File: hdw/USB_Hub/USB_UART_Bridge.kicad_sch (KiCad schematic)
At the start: 40 parts

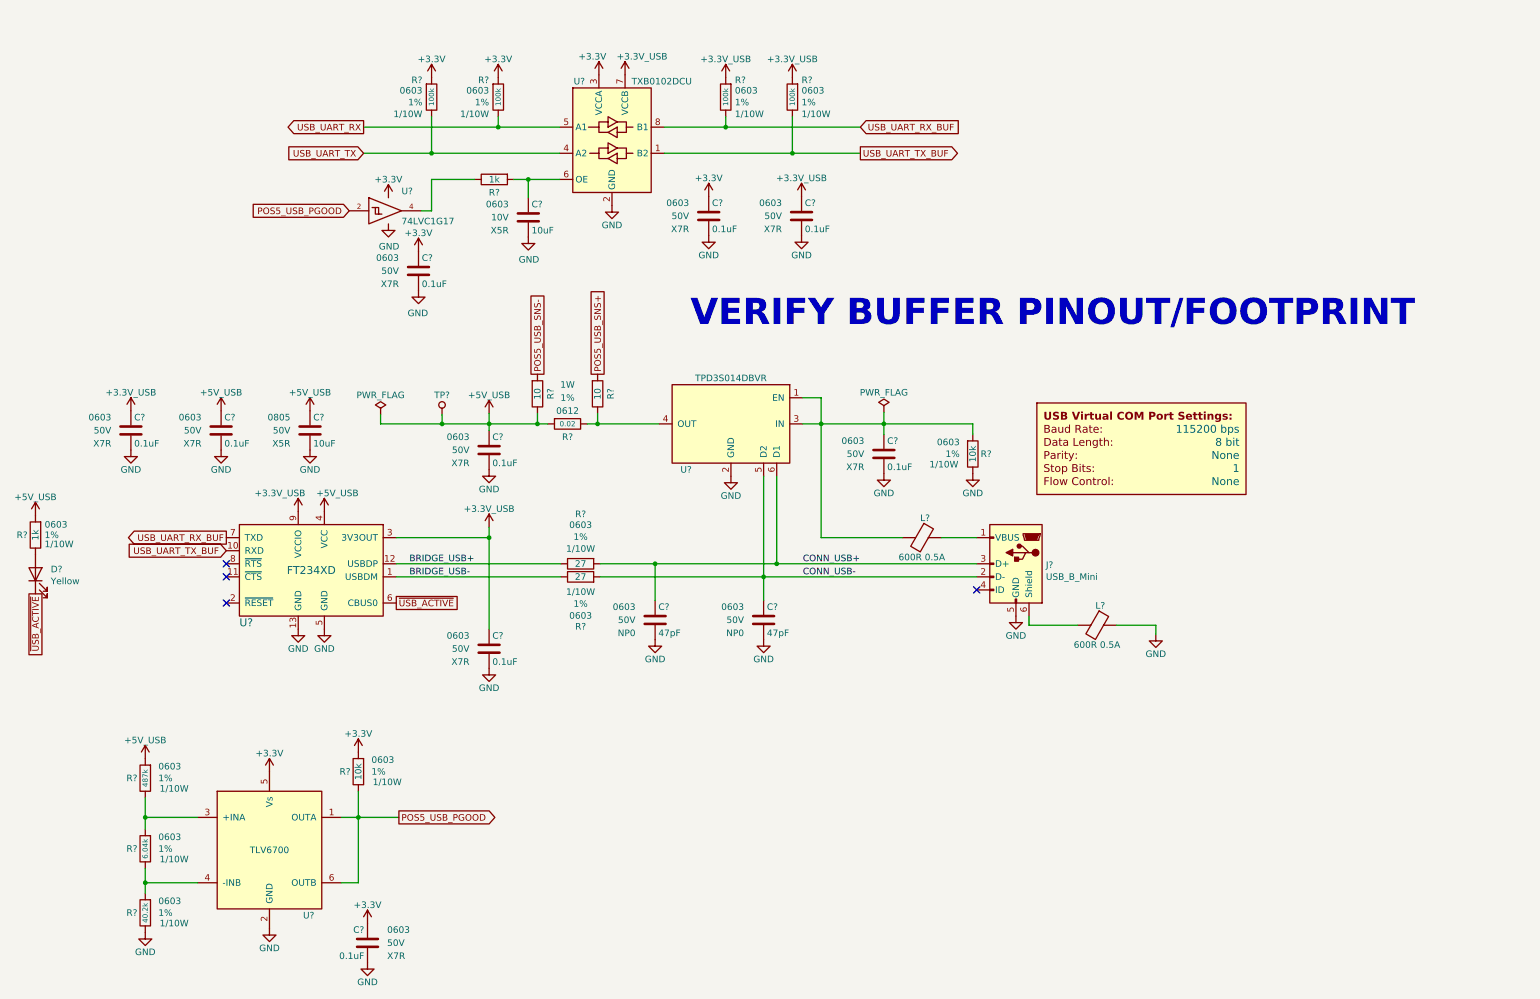
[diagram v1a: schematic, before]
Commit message: schematic progress
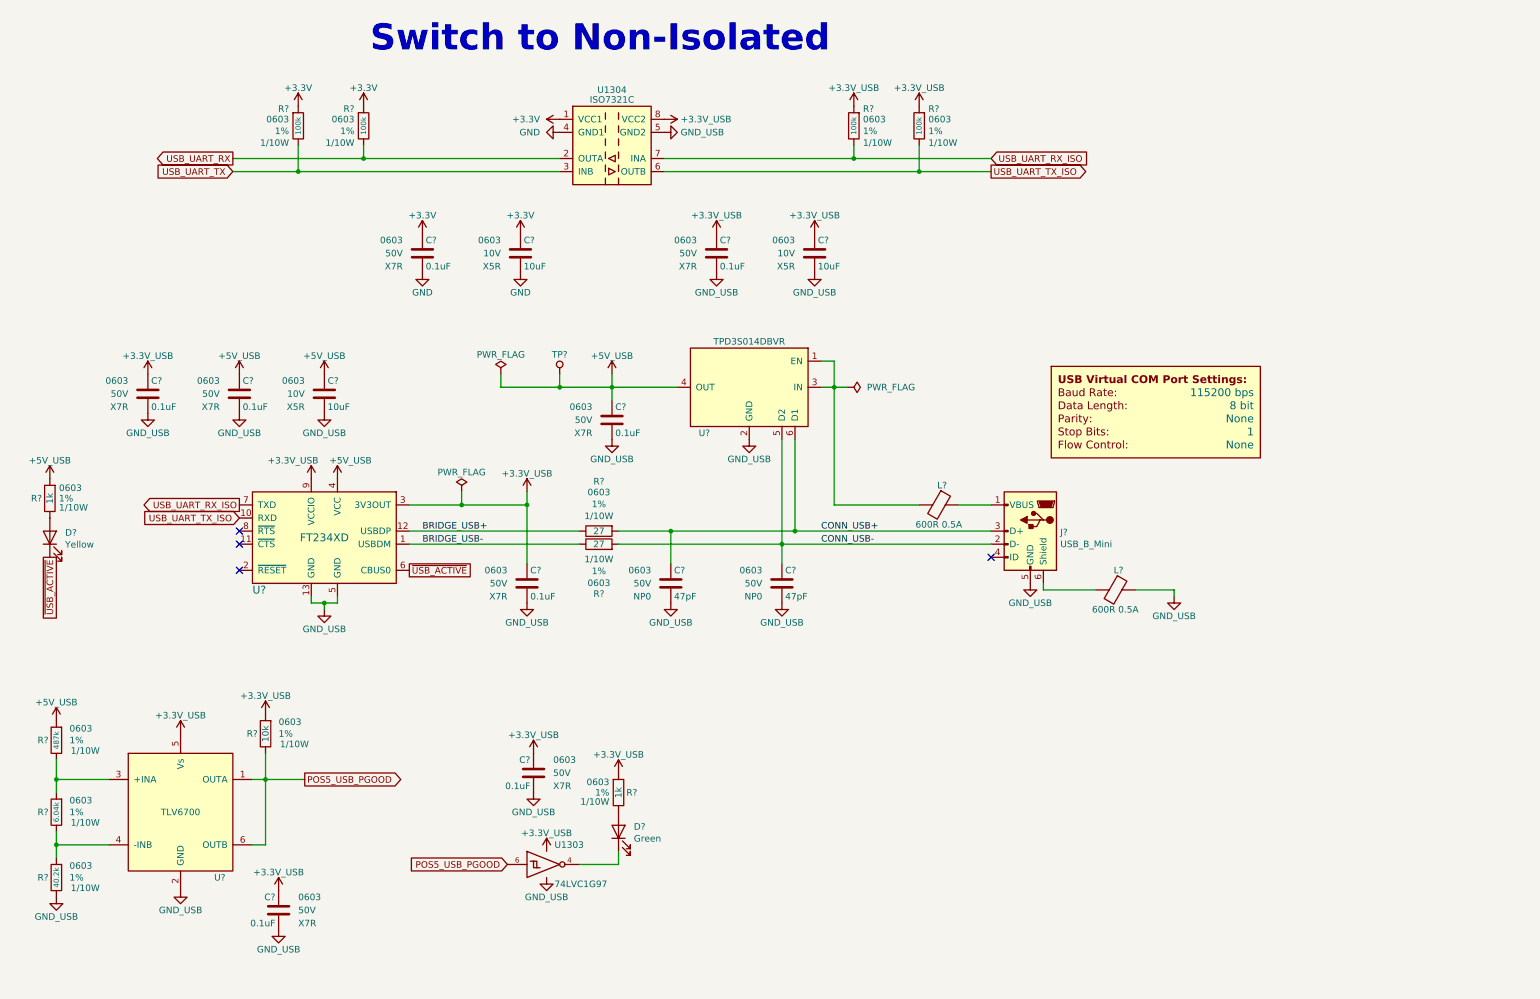
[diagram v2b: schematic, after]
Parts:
- removed C? (x2): 47pF, Capacitors_SMD:C_0603, symbol Custom_Library:C_Custom
- removed C? (x9): 0.1uF, Capacitors_SMD:C_0603, symbol Custom_Library:C_Custom
- removed C?: 10uF, Capacitors_SMD:C_0603, symbol Custom_Library:C_Custom
- removed C?: 10uF, Capacitors_SMD:C_0805, symbol Custom_Library:C_Custom
- removed D?: Yellow, LEDs:LED_0603, symbol Device:LED
- removed DOC?: COM_Port_Settings, symbol Custom_Library:COM_Port_Settings
- removed J?: USB_B_Mini, Connectors:USB_Mini-B, symbol Connector:USB_B_Mini
- removed L? (x2): 600R 0.5A, Inductors_SMD:L_0603, symbol Device:Ferrite_Bead
- removed R? (x2): 1k, Resistors_SMD:R_0603, symbol Custom_Library:R_Custom
- removed R? (x2): 27, Resistors_SMD:R_0603, symbol Custom_Library:R_Custom
- removed R?: 6.04k, Resistors_SMD:R_0603, symbol Custom_Library:R_Custom
- removed R?: 40.2k, Resistors_SMD:R_0603, symbol Custom_Library:R_Custom
- removed R?: 487k, Resistors_SMD:R_0603, symbol Custom_Library:R_Custom
- removed R? (x2): 10k, Resistors_SMD:R_0603, symbol Custom_Library:R_Custom
- removed R?: 0.02, Resistors_SMD:R_0612, symbol Custom_Library:R_Custom
- removed R? (x2): 10, Resistors_SMD:R_0603, symbol Custom_Library:R_Custom
- removed R? (x4): 100k, Resistors_SMD:R_0603, symbol Custom_Library:R_Custom
- removed TP?: TP, Custom Footprints Library:Test_Point, symbol Custom_Library:TP
- removed U?: FT234XD, Housings_DFN_QFN:DFN-12-1EP_3x3mm_Pitch0.45mm, symbol Custom_Library:FT234XD
- removed U?: TPD3S014DBVR, TO_SOT_Packages_SMD:SOT-23-6, symbol Custom_Library:TPD3S014DBVR
- removed U?: TLV6700, Package_TO_SOT_SMD:SOT-23-6, symbol Custom_Library:TLV6700
- removed U?: TXB0102DCU, Package_SO:VSSOP-8_2.4x2.1mm_P0.5mm, symbol Logic_LevelTranslator:TXB0102DCU
- removed U?: 74LVC1G17, TO_SOT_Packages_SMD:SOT-353_SC-70-5, symbol Custom_Library:74LVC1G17_Power
- added C? (x3): 10uF, Capacitors_SMD:C_0603, symbol Custom_Library:C_Custom
- added C? (x8): 0.1uF, Capacitors_SMD:C_0603, symbol Custom_Library:C_Custom
- added C? (x2): 47pF, Capacitors_SMD:C_0603, symbol Custom_Library:C_Custom
- added D?: Yellow, LEDs:LED_0603, symbol Device:LED
- added D?: Green, LEDs:LED_0603, symbol Device:LED
- added DOC?: COM_Port_Settings, symbol Custom_Library:COM_Port_Settings
- added J?: USB_B_Mini, Connectors:USB_Mini-B, symbol Connector:USB_B_Mini
- added L? (x2): 600R 0.5A, Inductors_SMD:L_0603, symbol Device:Ferrite_Bead
- added R? (x4): 100k, Resistors_SMD:R_0603, symbol Custom_Library:R_Custom
- added R?: 10k, Resistors_SMD:R_0603, symbol Custom_Library:R_Custom
- added R?: 487k, Resistors_SMD:R_0603, symbol Custom_Library:R_Custom
- added R?: 40.2k, Resistors_SMD:R_0603, symbol Custom_Library:R_Custom
- added R? (x2): 27, Resistors_SMD:R_0603, symbol Custom_Library:R_Custom
- added R?: 6.04k, Resistors_SMD:R_0603, symbol Custom_Library:R_Custom
- added R? (x2): 1k, Resistors_SMD:R_0603, symbol Custom_Library:R_Custom
- added TP?: TP, Custom Footprints Library:Test_Point, symbol Custom_Library:TP
- added U1303: 74LVC1G97, Package_TO_SOT_SMD:SOT-363_SC-70-6, symbol Custom Library:74LVC1G97_Power_NOT
- added U1304: ISO7321C, Package_SO:SOIC-8_3.9x4.9mm_P1.27mm, symbol Isolator:ISO7321C
- added U?: FT234XD, Housings_DFN_QFN:DFN-12-1EP_3x3mm_Pitch0.45mm, symbol Custom_Library:FT234XD
- added U?: TLV6700, Package_TO_SOT_SMD:SOT-23-6, symbol Custom_Library:TLV6700
- added U?: TPD3S014DBVR, TO_SOT_Packages_SMD:SOT-23-6, symbol Custom_Library:TPD3S014DBVR
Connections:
- net +3.3V: now also C?.1, C?.1, R?.1, R?.1, U1304.1 (VCC1)
- net +3.3V_USB: now also C?.1, C?.1, C?.1, C?.1, C?.1, C?.1, R?.1, R?.1, R?.1, R?.1, U1303.1 (VCC), U1303.5 (VCC), U1304.8 (VCC2), U?.3 (3V3OUT), U?.5 (Vs), U?.9 (VCCIO)
- net +5V_USB: now also C?.1, C?.1, C?.1, R?.1, R?.1, TP?.1 (TP), U?.4 (OUT), U?.4 (VCC)
- net BRIDGE_USB+: now also R?.2, U?.12 (USBDP)
- net BRIDGE_USB-: now also R?.2, U?.1 (USBDM)
- net CONN_USB+: now also C?.1, J?.3 (D+), R?.1, U?.6 (D1)
- net CONN_USB-: now also C?.1, J?.2 (D-), R?.1, U?.5 (D2)
- net GND: now also C?.2, C?.2, U1304.4 (GND1)
- net POS5_USB_PGOOD: now also R?.2, U1303.6, U?.1 (OUTA), U?.6 (OUTB)
- net USB_UART_RX: now also R?.2, U1304.2 (OUTA)
- net USB_UART_TX: now also R?.2, U1304.3 (INB)
- net ~{USB_ACTIVE}: now also D?.1 (K), U?.6 (CBUS0)
- new net: D?.1 (K), U1303.4
- new net: R?.1, R?.2, U?.3 (+INA)
- new net: J?.6 (Shield), L?.2
- new net: J?.1 (VBUS), L?.1
- new net: L?.2, U?.1 (EN), U?.3 (IN)
- new net: R?.1, R?.2, U?.4 (-INB)
- new net: D?.2 (A), R?.2 (x2)
- new net GND_USB: C?.2, C?.2, C?.2, C?.2, C?.2, C?.2, C?.2, C?.2, C?.2, C?.2, C?.2, J?.5 (GND), L?.1, R?.2, U1303.2 (GND), U1303.3 (GND), U1304.5 (GND2), U?.13 (GND), U?.2 (GND), U?.2 (GND), U?.5 (GND)
- new net USB_UART_RX_ISO: R?.2, U1304.7 (INA), U?.7 (TXD)
- new net USB_UART_TX_ISO: R?.2, U1304.6 (OUTB), U?.10 (RXD)
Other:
- note added: "Switch to Non-Isolated"
- note removed: "VERIFY BUFFER PINOUT/FOOTPRINT"
